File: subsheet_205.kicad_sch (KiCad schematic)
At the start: 34 parts, among them SW2 RESET, U10 MC68000_DIP_64_PHY, U36 74LS05_PHY, U37 LM556_DUAL_TIMER_PHY

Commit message: assigned footprint for all remaining standard passives
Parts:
- C105, C50, C55: footprint (none) -> Capacitor_THT:CP_Radial_D5.0mm_P2.50mm
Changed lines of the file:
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@@
       (effects (font (size 1.27 1.27)) (justify left))
     )
-    (property "Footprint" "" (id 2) (at 25.4 54.61 0)
+    (property "Footprint" "Capacitor_THT:CP_Radial_D5.0mm_P2.50mm" (id 2) (at 25.4 54.61 0)
       (effects (font (size 1.27 1.27)) hide)
     )
@@
       (effects (font (size 1.27 1.27)) (justify right))
     )
-    (property "Footprint" "" (id 2) (at 180.34 44.45 0)
+    (property "Footprint" "Capacitor_THT:CP_Radial_D5.0mm_P2.50mm" (id 2) (at 180.34 44.45 0)
       (effects (font (size 1.27 1.27)) hide)
     )
@@
       (effects (font (size 1.27 1.27)) (justify left))
     )
-    (property "Footprint" "" (id 2) (at 139.7 58.42 0)
-      (effects (font (size 1.27 1.27)) hide)
-    )
+    (property "Footprint" "Capacitor_THT:CP_Radial_D5.0mm_P2.50mm" (id 2) (at 139.7 58.42 0)
+      (effects (font (size 1.27 1.27)) hide)
+    )

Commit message: done assigning footprints
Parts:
- SW2: footprint (none) -> atari-interconnect:switch-spdt-momentary-action_Reset_pushbutton
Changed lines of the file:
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@@
     )
     (property "Value" "RESET" (id 1) (at 29.21 84.074 0))
-    (property "Footprint" "" (id 2) (at 29.21 77.47 0)
+    (property "Footprint" "atari-interconnect:switch-spdt-momentary-action_Reset_pushbutton" (id 2) (at 29.21 77.47 0)
       (effects (font (size 1.27 1.27)) hide)
     )

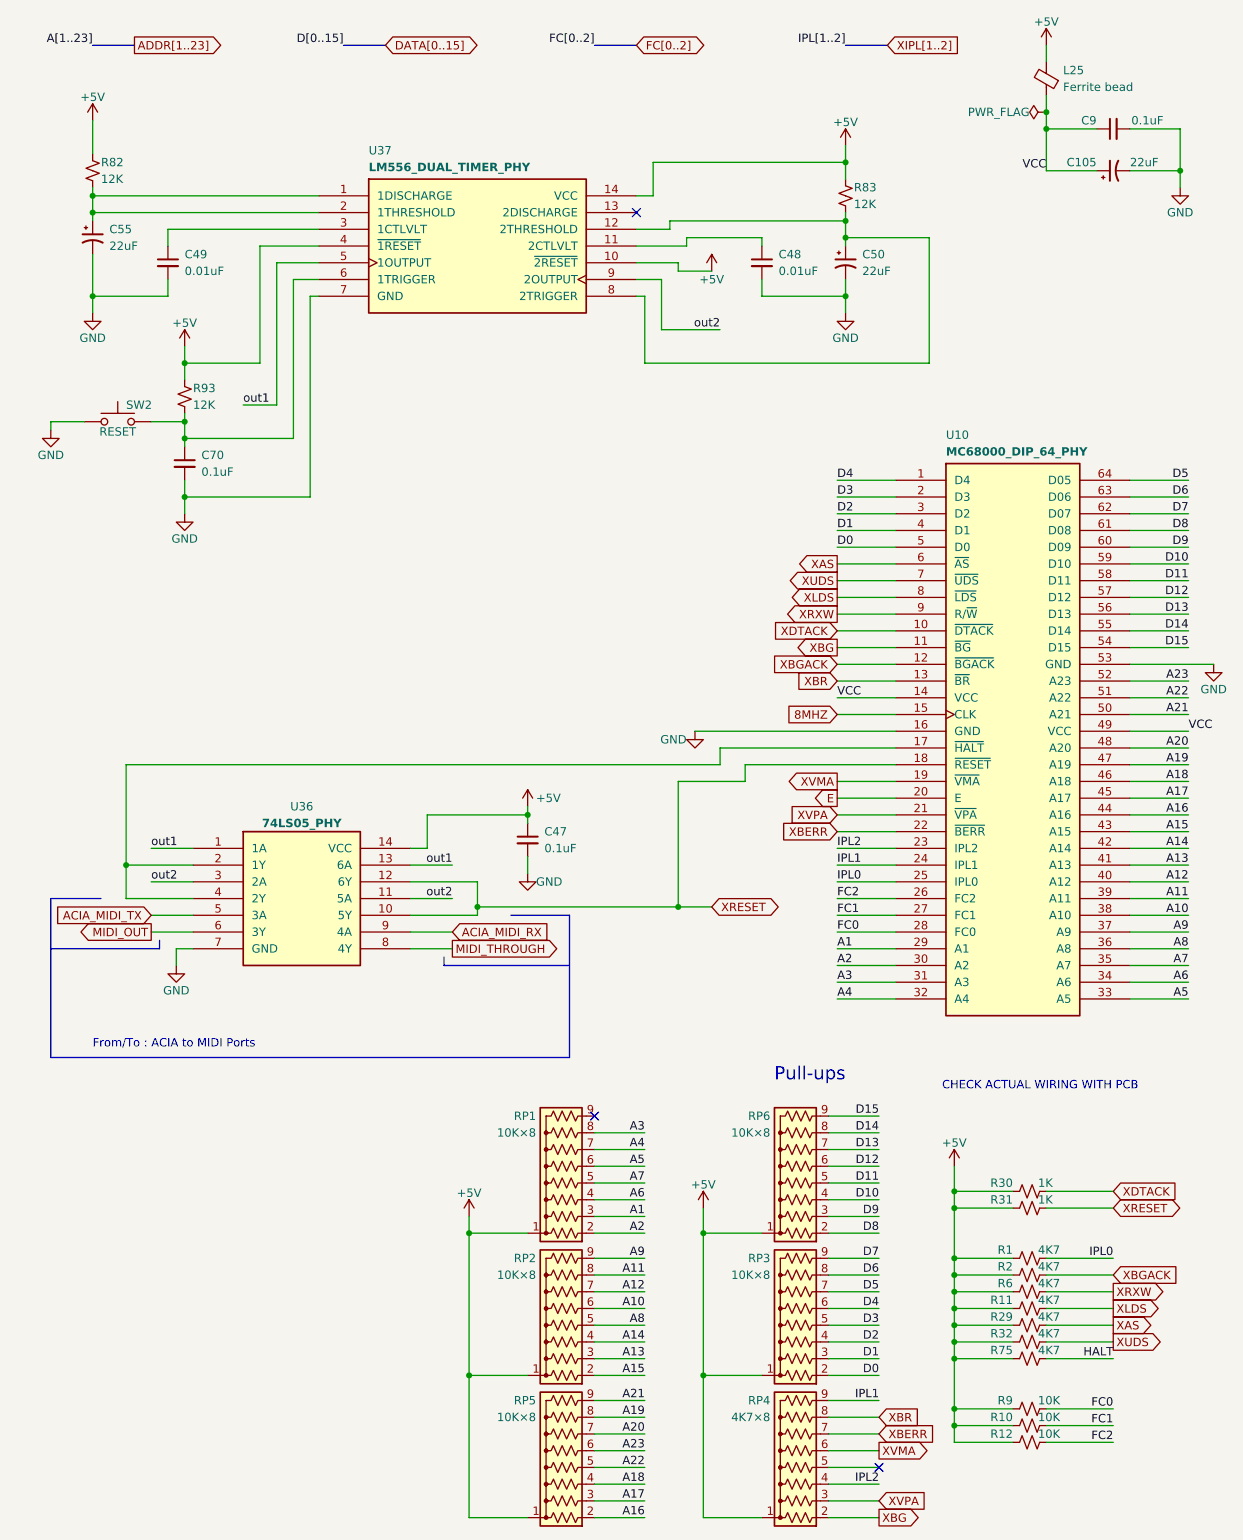
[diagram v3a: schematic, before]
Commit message: fixed all RPx : use 9-bussed resistor networks, fixed wiring
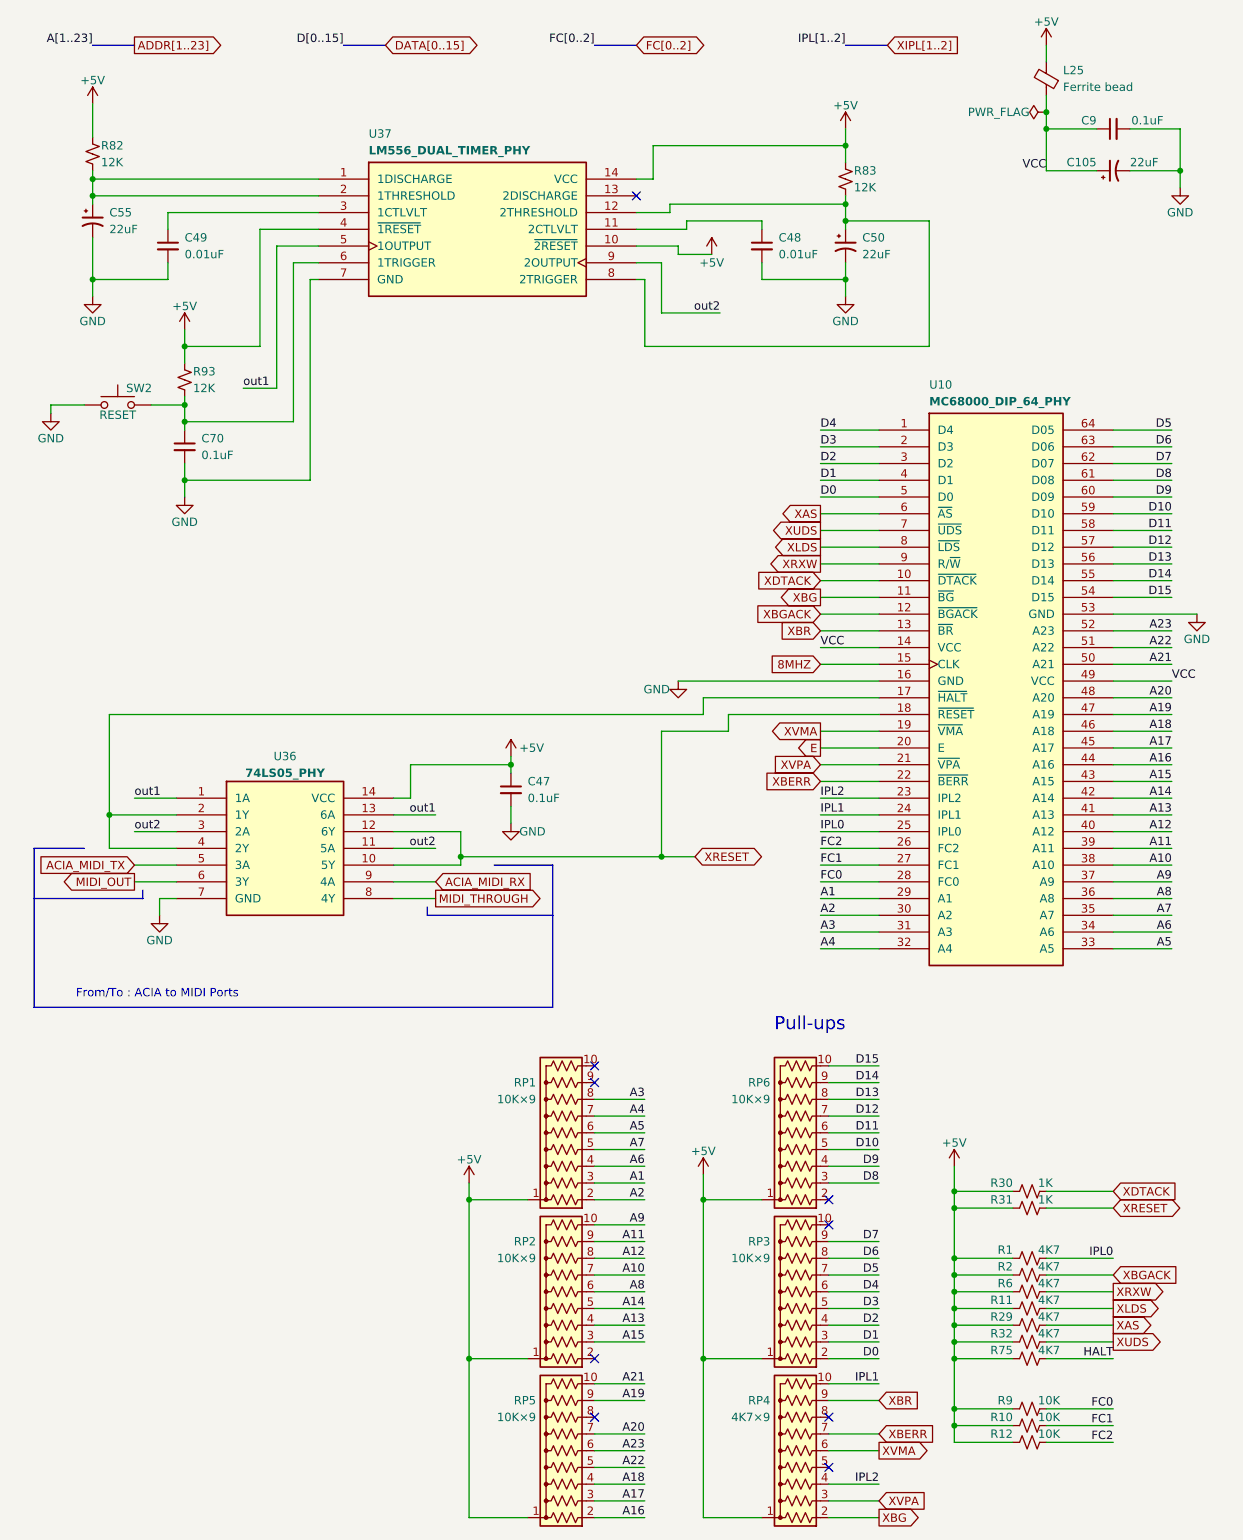
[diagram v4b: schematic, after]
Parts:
- RP1, RP2, RP3, RP5, RP6: value 10K×8 -> 10K×9; footprint Resistor_THT:R_Array_SIP9 -> Resistor_THT:R_Array_SIP10; symbol Device:R_Network08_US -> Device:R_Network09_US
- RP4: value 4K7×8 -> 4K7×9; footprint Resistor_THT:R_Array_SIP9 -> Resistor_THT:R_Array_SIP10; symbol Device:R_Network08_US -> Device:R_Network09_US
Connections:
- net A10: now also RP2.7 (R6); no longer RP2.6 (R5)
- net A11: now also RP2.9 (R8); no longer RP2.8 (R7)
- net A12: now also RP2.8 (R7); no longer RP2.7 (R6)
- net A13: now also RP2.4 (R3); no longer RP2.3 (R2)
- net A14: now also RP2.5 (R4); no longer RP2.4 (R3)
- net A15: now also RP2.3 (R2); no longer RP2.2 (R1)
- net A19: now also RP5.9 (R8); no longer RP5.8 (R7)
- net A21: now also RP5.10 (R9); no longer RP5.9 (R8)
- net A8: now also RP2.6 (R5); no longer RP2.5 (R4)
- net A9: now also RP2.10 (R9); no longer RP2.9 (R8)
- net D10: now also RP6.5 (R4); no longer RP6.4 (R3)
- net D11: now also RP6.6 (R5); no longer RP6.5 (R4)
- net D12: now also RP6.7 (R6); no longer RP6.6 (R5)
- net D13: now also RP6.8 (R7); no longer RP6.7 (R6)
- net D14: now also RP6.9 (R8); no longer RP6.8 (R7)
- net D15: now also RP6.10 (R9); no longer RP6.9 (R8)
- net D8: now also RP6.3 (R2); no longer RP6.2 (R1)
- net D9: now also RP6.4 (R3); no longer RP6.3 (R2)
- net IPL1: now also RP4.10 (R9); no longer RP4.9 (R8)
- net XBR: now also RP4.9 (R8); no longer RP4.8 (R7)
- no-connect marks 3 -> 9
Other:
- note removed: "CHECK ACTUAL WIRING WITH PCB"
- moved on the sheet: C47, C48, C49, C50, C55, C70, R82, R83, R93, SW2, U10, U36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
